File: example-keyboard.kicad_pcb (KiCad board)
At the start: 2 copper layers, 68.6 x 54.6 mm, 10 parts, among them SW1 SW_Push, U1 Elite-C

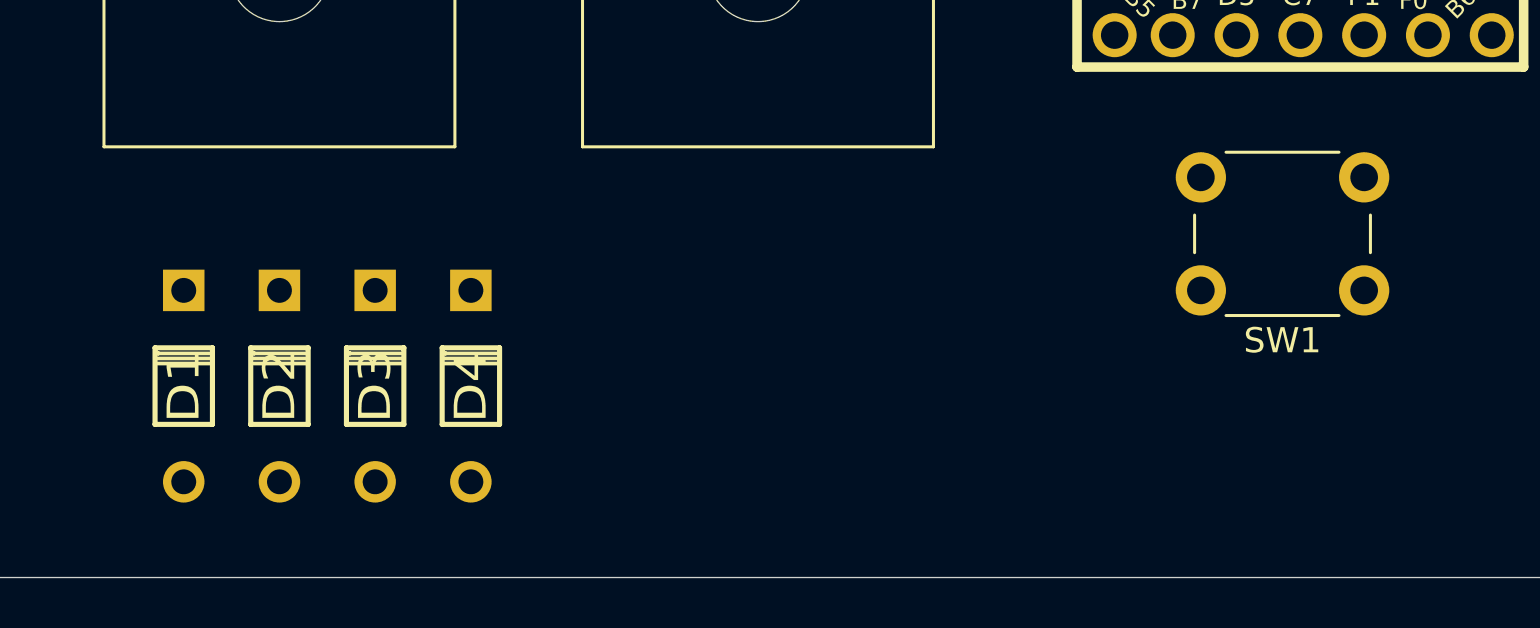
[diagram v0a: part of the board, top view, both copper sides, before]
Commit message: better layout
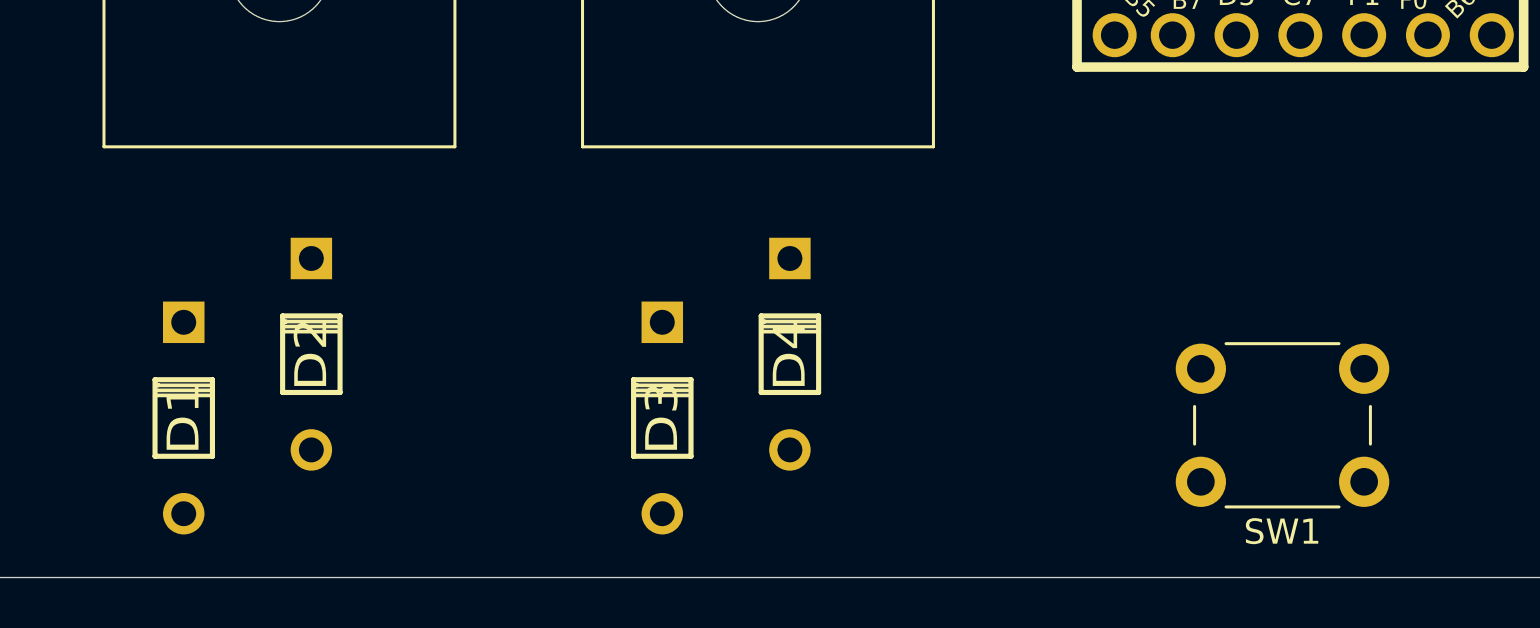
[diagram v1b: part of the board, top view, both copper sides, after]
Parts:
- moved D4 12.8 mm to (97.8, 92.7)
- moved D3 11.5 mm to (92.7, 95.2)
- moved SW1 7.62 mm to (120.7, 97.8)
- moved D2 1.80 mm to (78.7, 92.7)
- moved D1 1.27 mm to (73.7, 95.2)
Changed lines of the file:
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@@
   )
   (module Button_Switch_THT:SW_PUSH_6mm_H7.3mm (layer F.Cu)
-    (at 120.65 90.17 180)
+    (at 120.65 97.79 180)
     (descr "tactile push button, 6x6mm e.g. PHAP33xx series, height=7.3mm")
     (tags "tact sw push 6mm")
@@
   )
   (module Keebio-Parts:Diode (layer F.Cu)
-    (at 85.09 93.98 90)
+    (at 97.79 92.71 90)
     (fp_text reference D4 (at 0 0 90) (layer F.SilkS)
       (effects (font (size 1.27 1.524) (thickness 0.2032)))
@@
   )
   (module Keebio-Parts:Diode (layer F.Cu)
-    (at 81.28 93.98 90)
+    (at 92.71 95.25 90)
     (fp_text reference D3 (at 0 0 90) (layer F.SilkS)
       (effects (font (size 1.27 1.524) (thickness 0.2032)))
@@
   )
   (module Keebio-Parts:Diode (layer F.Cu)
-    (at 77.47 93.98 90)
+    (at 78.74 92.71 90)
     (fp_text reference D2 (at 0 0 90) (layer F.SilkS)
       (effects (font (size 1.27 1.524) (thickness 0.2032)))
@@
   )
   (module Keebio-Parts:Diode (layer F.Cu)
-    (at 73.66 93.98 90)
+    (at 73.66 95.25 90)
     (fp_text reference D1 (at 0 0 90) (layer F.SilkS)
       (effects (font (size 1.27 1.524) (thickness 0.2032)))
